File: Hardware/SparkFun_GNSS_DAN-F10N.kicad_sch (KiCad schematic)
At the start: 52 parts, among them J1 USB_C_Receptacle, J2 Conn_01x06, J4 U.FL, J5 Conn_01x08, U1 DT1042-04SO, U3 RT9080-3.3, U4 CH340C, U6 DAN-F10N

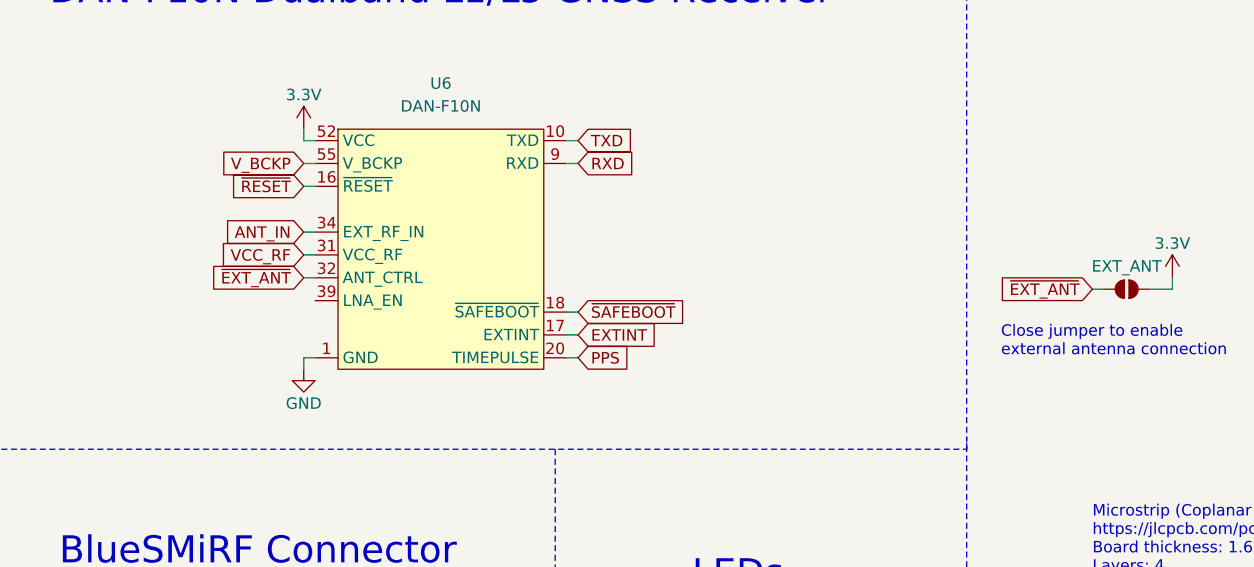
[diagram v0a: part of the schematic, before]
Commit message: Add panel
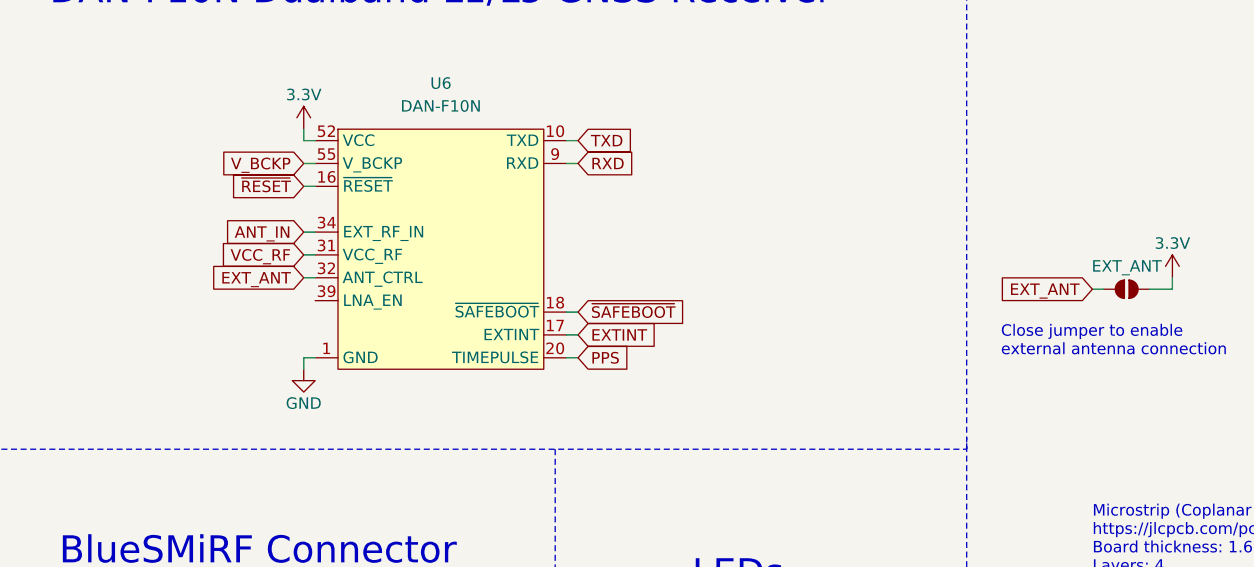
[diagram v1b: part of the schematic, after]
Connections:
- net ~{EXT_ANT} renamed EXT_ANT
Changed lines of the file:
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@@
 		)
 	)
-	(global_label "~{EXT_ANT}"
+	(global_label "EXT_ANT"
 		(shape input)
 		(at 250.19 124.46 180)
@@
 		)
 	)
-	(global_label "~{EXT_ANT}"
+	(global_label "EXT_ANT"
 		(shape input)
 		(at 162.56 123.19 180)
